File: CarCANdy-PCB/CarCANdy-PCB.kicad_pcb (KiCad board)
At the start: 2 copper layers, 40 parts, among them J1 8P8C_Shielded, J2 Power, K1 IM06TS, T1 NTD5867NL, U2 ESP32-C3_SUPERMINI_TH, U3 SN65HVD233DR, U4 SN65HVD233DR, U5 SN65HVD233DR, U6 Teensy4.1, U7 LTV-817S

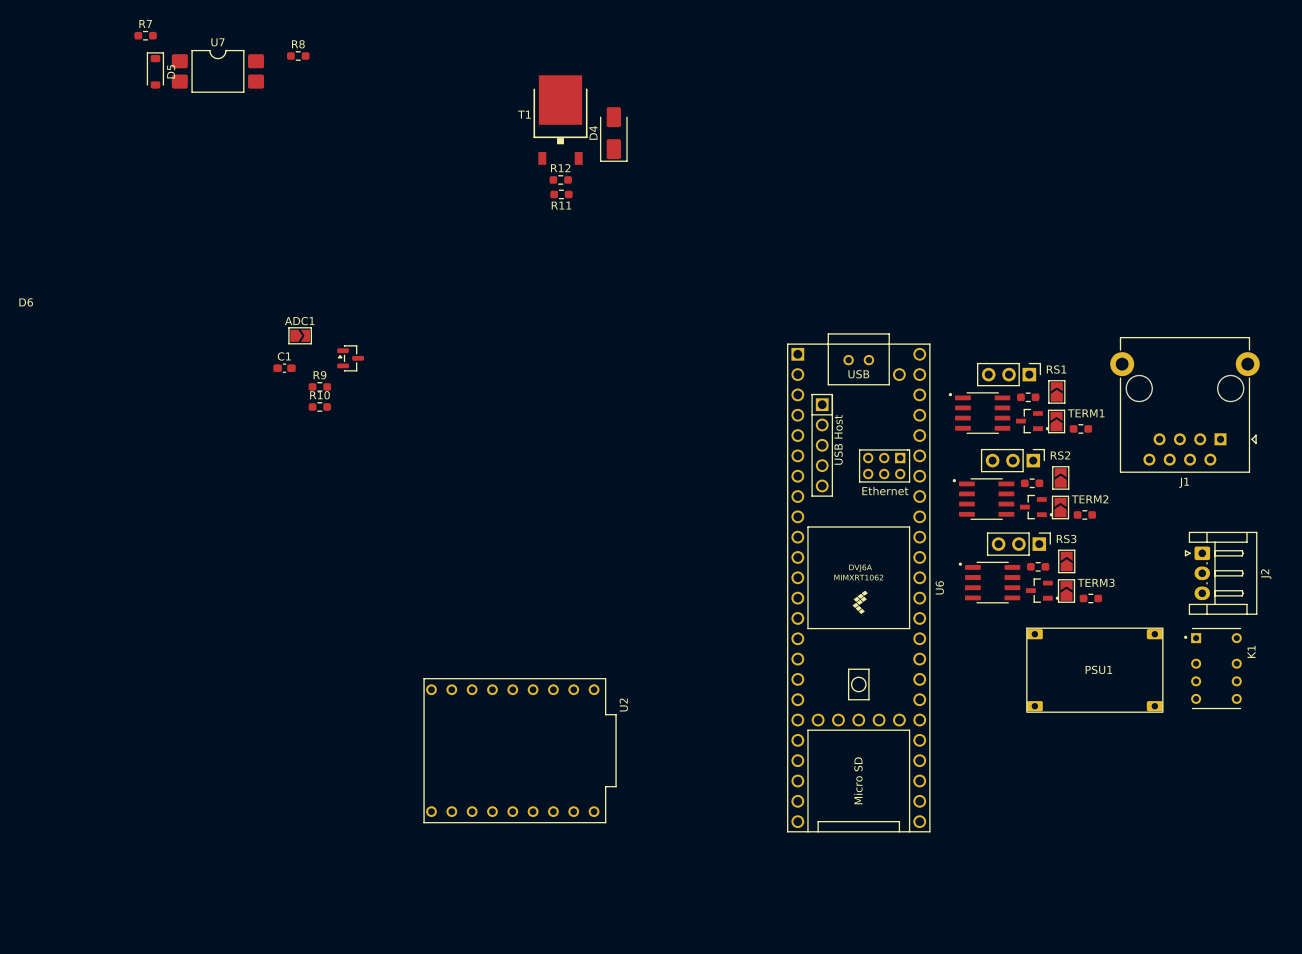
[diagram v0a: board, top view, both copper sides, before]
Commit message: added to PCB
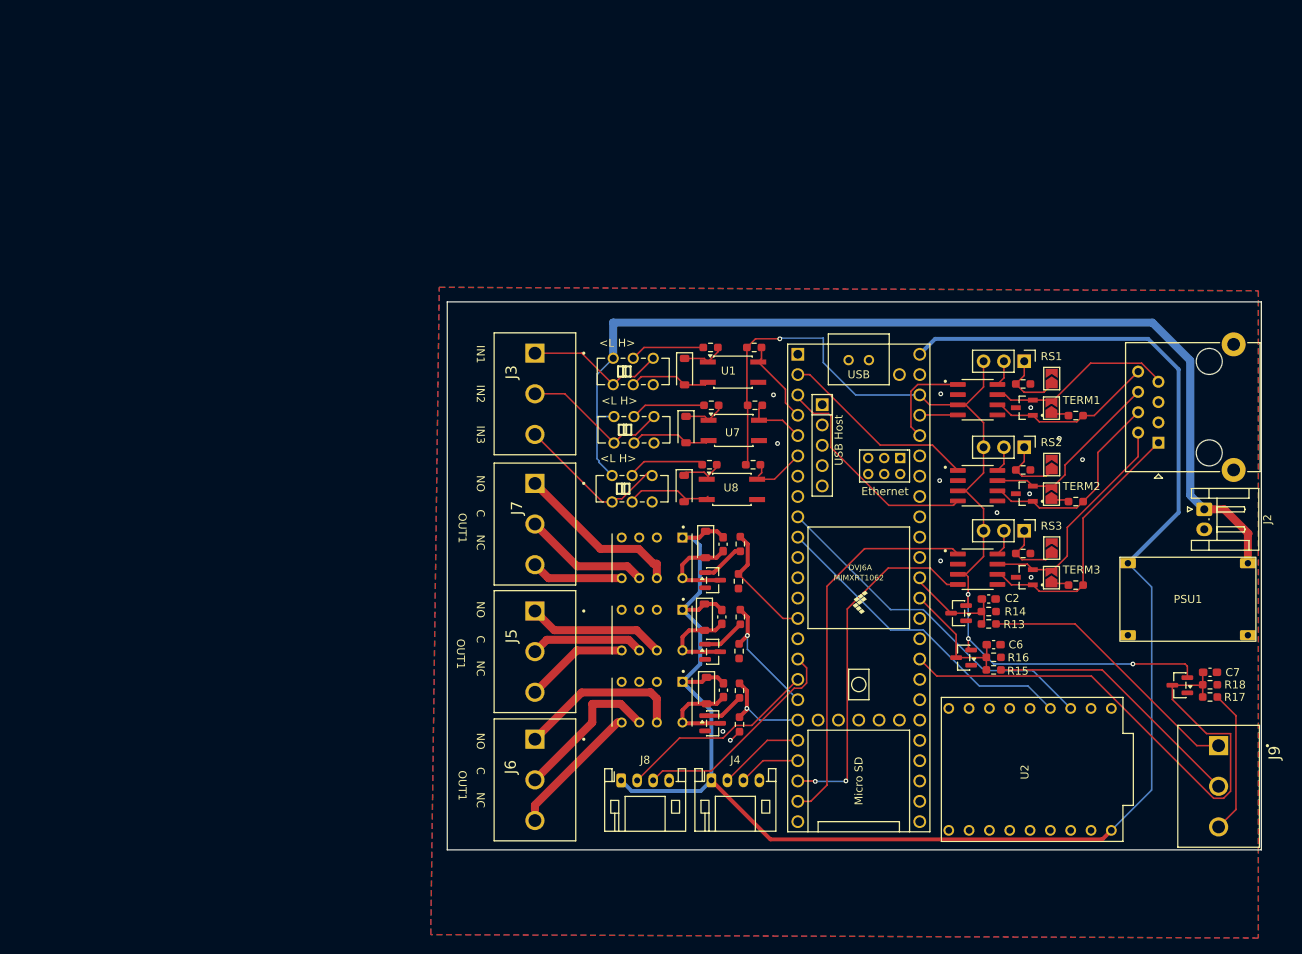
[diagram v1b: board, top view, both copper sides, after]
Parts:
- removed ADC1: RS, Jumper:SolderJumper-2_P1.3mm_Open_TrianglePad1.0x1.5mm
- removed C1: 100nF, Capacitor_SMD:C_0603_1608Metric_Pad1.08x0.95mm_HandSolder
- removed D4: SS14, Diode_SMD:D_SMA
- removed D6: BAT54S, Package_TO_SOT_SMD:SOT-23
- removed K1: IM06TS, IM06:RELAY_IM06TS
- removed R10: 33K, Resistor_SMD:R_0603_1608Metric_Pad0.98x0.95mm_HandSolder
- removed R11: 100, Resistor_SMD:R_0603_1608Metric_Pad0.98x0.95mm_HandSolder
- removed R12: 47k, Resistor_SMD:R_0603_1608Metric_Pad0.98x0.95mm_HandSolder
- removed R9: 180K, Resistor_SMD:R_0603_1608Metric_Pad0.98x0.95mm_HandSolder
- removed T1: NTD5867NL, NTD5867NL:DPACK
- added C2: 100nF, Capacitor_SMD:C_0603_1608Metric_Pad1.08x0.95mm_HandSolder, F.Cu at (122.4, 86.4)
- added C3: 100nF, Capacitor_SMD:C_0603_1608Metric_Pad1.08x0.95mm_HandSolder, F.Cu at (89.2, 79.6)
- added C4: 100nF, Capacitor_SMD:C_0603_1608Metric_Pad1.08x0.95mm_HandSolder, F.Cu at (89.0, 88.6)
- added C5: 100nF, Capacitor_SMD:C_0603_1608Metric_Pad1.08x0.95mm_HandSolder, F.Cu at (89.2, 97.8)
- added C6: 100nF, Capacitor_SMD:C_0603_1608Metric_Pad1.08x0.95mm_HandSolder, F.Cu at (123.0, 92.1)
- added C7: 100nF, Capacitor_SMD:C_0603_1608Metric_Pad1.08x0.95mm_HandSolder, F.Cu at (150.0, 95.6)
- added D10: 1N4148W, Diode_SMD:D_SOD-123, F.Cu at (84.3, 72.6)
- added D11: 1N4148W, Diode_SMD:D_SOD-123, F.Cu at (86.8, 88.7)
- added D12: 1N4148W, Diode_SMD:D_SOD-123, F.Cu at (87.1, 97.8)
- added D13: BAT54S, Package_TO_SOT_SMD:SOT-23, F.Cu at (119.2, 93.7)
- added D14: BAT54S, Package_TO_SOT_SMD:SOT-23, F.Cu at (146.3, 97.2)
- added D7: BAT54S, Package_TO_SOT_SMD:SOT-23, F.Cu at (118.6, 88.2)
- added D8: 1N4148W, Diode_SMD:D_SOD-123, F.Cu at (87.0, 79.6)
- added D9: 1N4148W, Diode_SMD:D_SOD-123, F.Cu at (84.5, 65.2)
- added J3: TB004-508-03BE, TB004-508-03BE:CUI_TB004-508-03BE, F.Cu at (65.7, 55.7)
- added J4: AUART1, Connector_JST:JST_PH_S4B-PH-K_1x04_P2.00mm_Horizontal, F.Cu at (87.7, 109.1)
- added J5: TB004-508-03BE, TB004-508-03BE:CUI_TB004-508-03BE, F.Cu at (65.7, 87.9)
- added J6: TB004-508-03BE, TB004-508-03BE:CUI_TB004-508-03BE, F.Cu at (65.7, 103.9)
- added J7: TB004-508-03BE, TB004-508-03BE:CUI_TB004-508-03BE, F.Cu at (65.7, 72.0)
- added J8: AUART1, Connector_JST:JST_PH_S4B-PH-K_1x04_P2.00mm_Horizontal, F.Cu at (76.4, 109.1)
- added J9: TB004-508-03BE, TB004-508-03BE:CUI_TB004-508-03BE, F.Cu at (151.1, 104.7)
- added K3: IM02, IM06:RELAY_IM06TS, F.Cu at (80.3, 81.3)
- added K4: IM02, IM06:RELAY_IM06TS, F.Cu at (80.3, 90.3)
- added K5: IM02, IM06:RELAY_IM06TS, F.Cu at (80.3, 99.3)
- added Q1: AO3400A, Package_TO_SOT_SMD:SOT-23, F.Cu at (87.9, 84.0)
- added Q2: AO3400A, Package_TO_SOT_SMD:SOT-23, F.Cu at (87.9, 93.0)
- added Q3: AO3400A, Package_TO_SOT_SMD:SOT-23, F.Cu at (87.9, 101.9)
- added R13: 22K, Resistor_SMD:R_0603_1608Metric_Pad0.98x0.95mm_HandSolder, F.Cu at (122.4, 89.5)
- added R14: 33K, Resistor_SMD:R_0603_1608Metric_Pad0.98x0.95mm_HandSolder, F.Cu at (122.4, 88.0)
- added R15: 22K, Resistor_SMD:R_0603_1608Metric_Pad0.98x0.95mm_HandSolder, F.Cu at (123.0, 95.3)
- added R16: 33K, Resistor_SMD:R_0603_1608Metric_Pad0.98x0.95mm_HandSolder, F.Cu at (123.0, 93.7)
- added R17: 22K, Resistor_SMD:R_0603_1608Metric_Pad0.98x0.95mm_HandSolder, F.Cu at (150.0, 98.7)
- added R18: 33K, Resistor_SMD:R_0603_1608Metric_Pad0.98x0.95mm_HandSolder, F.Cu at (150.0, 97.1)
- added R19: 100, Resistor_SMD:R_0603_1608Metric_Pad0.98x0.95mm_HandSolder, F.Cu at (91.3, 79.5)
- added R20: 47K, Resistor_SMD:R_0603_1608Metric_Pad0.98x0.95mm_HandSolder, F.Cu at (91.1, 84.2)
- added R21: 2.2K, Resistor_SMD:R_0603_1608Metric_Pad0.98x0.95mm_HandSolder, F.Cu at (87.7, 62.2)
- added R22: 10k, Resistor_SMD:R_0603_1608Metric_Pad0.98x0.95mm_HandSolder, F.Cu at (93.2, 62.2)
- added R23: 2.2K, Resistor_SMD:R_0603_1608Metric_Pad0.98x0.95mm_HandSolder, F.Cu at (87.5, 69.6)
- added R24: 10k, Resistor_SMD:R_0603_1608Metric_Pad0.98x0.95mm_HandSolder, F.Cu at (92.9, 69.6)
- added R25: 100, Resistor_SMD:R_0603_1608Metric_Pad0.98x0.95mm_HandSolder, F.Cu at (91.3, 88.6)
- added R26: 47K, Resistor_SMD:R_0603_1608Metric_Pad0.98x0.95mm_HandSolder, F.Cu at (91.2, 92.9)
- added R27: 100, Resistor_SMD:R_0603_1608Metric_Pad0.98x0.95mm_HandSolder, F.Cu at (91.2, 97.8)
- added R28: 47K, Resistor_SMD:R_0603_1608Metric_Pad0.98x0.95mm_HandSolder, F.Cu at (91.2, 102.1)
- added SW2: JS202011CQN, JS202011CQN:JS202011CQN, F.Cu at (77.9, 58.0)
- added SW3: JS202011CQN, JS202011CQN:JS202011CQN, F.Cu at (78.0, 65.2)
- added SW4: JS202011CQN, JS202011CQN:JS202011CQN, F.Cu at (77.8, 72.6)
- added U1: LTV-357T, Package_SO:SO-4_4.4x3.6mm_P2.54mm, F.Cu at (90.4, 58.0)
- added U8: LTV-357T, Package_SO:SO-4_4.4x3.6mm_P2.54mm, F.Cu at (90.3, 72.7)
- J2: footprint Connector_JST:JST_EH_S3B-EH_1x03_P2.50mm_Horizontal -> Connector_JST:JST_EH_S2B-EH_1x02_P2.50mm_Horizontal
- U7: value LTV-817S -> LTV-357T; footprint Package_DIP:SMDIP-4_W9.53mm -> Package_SO:SO-4_4.4x3.6mm_P2.54mm
- moved R7 80.7 mm to (87.6, 55.0)
- moved U7 78.6 mm to (90.5, 65.3)
- moved D5 76.0 mm to (84.4, 58.0)
- moved R8 67.6 mm to (93.1, 55.0), turned to 180 degrees
- moved U2 64.7 mm to (127.8, 107.7)
- moved PSU1 14.6 mm to (147.3, 86.4)
- moved J1 7.77 mm to (143.6, 66.9), turned to 90 degrees
- moved J2 5.51 mm to (149.3, 75.2)
- moved R6 2.51 mm to (126.7, 80.7)
- moved D3 2.51 mm to (126.8, 83.7)
- moved JP9 2.51 mm to (126.8, 77.9)
- moved R5 2.51 mm to (133.3, 84.7)
- moved RS3 2.51 mm to (130.2, 80.0)
- moved TERM3 2.51 mm to (130.2, 83.7)
- moved U5 2.51 mm to (121.0, 82.7)
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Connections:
- D5 pad 2: GND -> Net-(D5-A)
- J2 pad 1: 12v_CONST -> +12V
- J2 pad 2: 12v_IGN -> GND
- R7 pad 1: 12V_INPUT -> Net-(SW2A-B)
- R8 pad 1: GPIO -> GPIO_IN1
- U6 pad 1: unconnected-(U6-GND-Pad1) -> GND
- U6 pad 14: unconnected-(U6-12_MISO_MQSL-Pad14) -> GPIO_OUT1
- U6 pad 16: unconnected-(U6-24_A10_TX6_SCL2-Pad16) -> ATX2
- U6 pad 17: unconnected-(U6-25_A11_RX6_SDA2-Pad17) -> ARX2
- U6 pad 18: unconnected-(U6-26_A12_MOSI1-Pad18) -> GPIO_OUT2
- U6 pad 19: unconnected-(U6-27_A13_SCK1-Pad19) -> GPIO_OUT3
- U6 pad 20: unconnected-(U6-28_RX7-Pad20) -> ARX1
- U6 pad 21: unconnected-(U6-29_TX7-Pad21) -> ATX1
- U6 pad 33: unconnected-(U6-41_A17-Pad33) -> ADC3
- U6 pad 34: unconnected-(U6-GND-Pad34) -> GND
- U6 pad 36: unconnected-(U6-14_A0_TX3_SPDIF_OUT-Pad36) -> ADC2
- U6 pad 37: unconnected-(U6-15_A1_RX3_SPDIF_IN-Pad37) -> ADC1
- U6 pad 4: unconnected-(U6-2_OUT2-Pad4) -> GPIO_IN1
- U6 pad 47: unconnected-(U6-GND-Pad47) -> GND
- U6 pad 5: unconnected-(U6-3_LRCLK2-Pad5) -> GPIO_IN2
- U6 pad 52: unconnected-(U6-GND-Pad52) -> GND
- U6 pad 6: unconnected-(U6-4_BCLK2-Pad6) -> GPIO_IN3
- U7 pad 1: Net-(D5-K) -> Net-(D9-K)
- U7 pad 2: GND -> Net-(D9-A)
- U7 pad 4: GPIO -> GPIO_IN2
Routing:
- net +5V: track 0.00 -> 217.3 mm
- net +12V: track 0.00 -> 126.9 mm
- net +3.3V: track 0.00 -> 122.6 mm, vias 0 -> 4
- net ADC3: track 0.00 -> 71.4 mm
- net CAN3_TX: track 0.00 -> 47.9 mm
- net CAN3_RX: track 0.00 -> 44.4 mm, vias 0 -> 2
- net T_RX->E_TX: track 0.00 -> 44.0 mm
- net T_TX->E_RX: track 0.00 -> 40.4 mm
- net 5V_SIG1: track 0.00 -> 34.1 mm
- net CAN3_L: track 0.00 -> 33.6 mm
- net 5V_SIG2: track 0.00 -> 33.2 mm
- net CAN3_H: track 0.00 -> 29.1 mm
- net CAN2_RX: track 0.00 -> 28.5 mm
- net ATX2: track 0.00 -> 27.7 mm
- net CAN2_L: track 0.00 -> 25.9 mm
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- added copper zone on B.Cu, net GND
- added copper zone on F.Cu, net GND
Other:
- board outline added: 101.8 x 68.5 mm
- board text added: "<L H>"
- board text added: "IN1"
- board text added: "IN2"
- board text added: "IN3"
- board text added: "NO C NC"
- board text added: "OUT1"
